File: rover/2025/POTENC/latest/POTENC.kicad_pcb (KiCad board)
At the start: 4 copper layers, 20 x 23.1 mm, 4 parts, among them J1 POT, J2 Conn_01x06_Socket, J3 RJ50-SS-641010-A-NF-A111

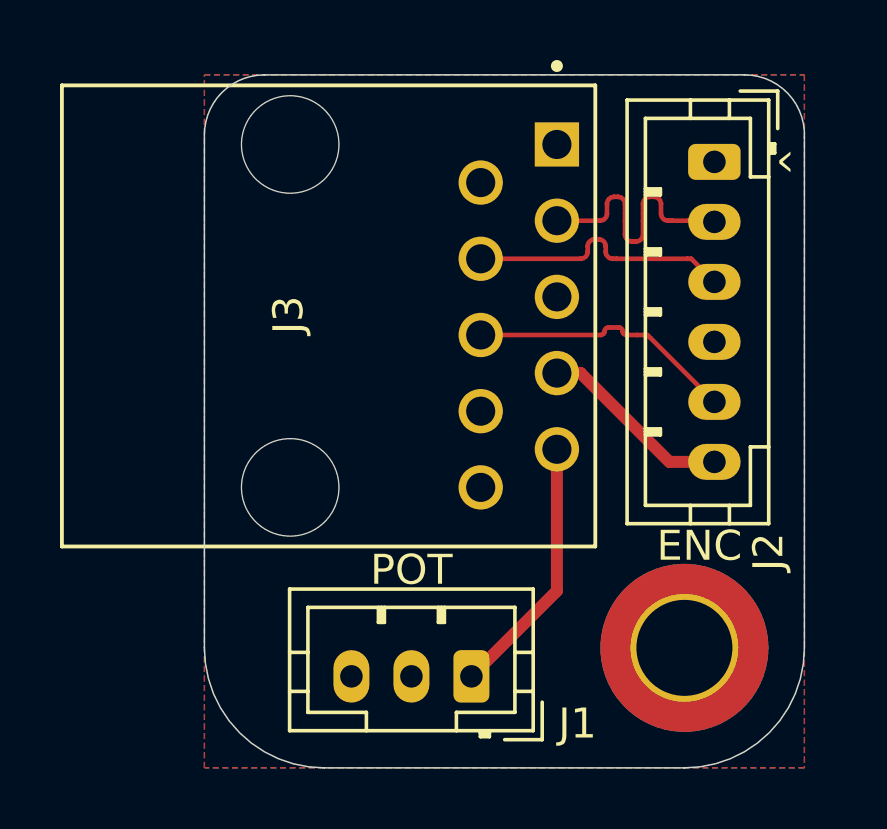
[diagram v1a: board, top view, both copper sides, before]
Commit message: ARM-JL REV0 done
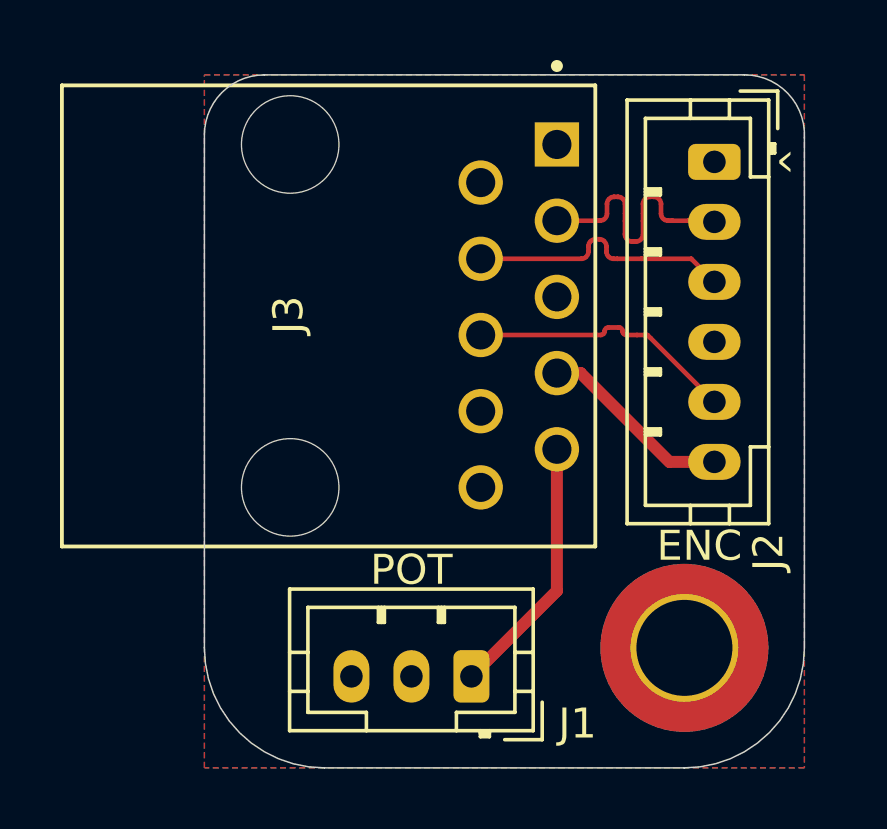
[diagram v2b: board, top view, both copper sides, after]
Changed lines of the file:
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@@
 	)
 	(segment
-		(start 54.28766 38.84)
-		(end 54.40766 38.84)
-		(width 0.1565)
-		(layer "F.Cu")
-		(net 5)
-	)
-	(segment
-		(start 54.04766 38.428531)
-		(end 54.04766 38.6)
-		(width 0.1565)
-		(layer "F.Cu")
-		(net 5)
-	)
-	(segment
-		(start 56.778149 38.84)
-		(end 56.901 38.84)
-		(width 0.1565)
-		(layer "F.Cu")
-		(net 5)
-	)
-	(segment
-		(start 53.68766 38.188531)
-		(end 53.80766 38.188531)
+		(start 54.432799 38.84)
+		(end 55.237661 38.84)
+		(width 0.1565)
+		(layer "F.Cu")
+		(net 5)
+	)
+	(segment
+		(start 49.881 38.84)
+		(end 53.232799 38.84)
 		(width 0.1565)
 		(layer "F.Cu")
@@
 	)
 	(segment
-		(start 54.40766 38.84)
-		(end 56.778149 38.84)
-		(width 0.1565)
-		(layer "F.Cu")
-		(net 5)
-	)
-	(segment
-		(start 53.44766 38.6)
-		(end 53.44766 38.428531)
-		(width 0.1565)
-		(layer "F.Cu")
-		(net 5)
-	)
-	(segment
-		(start 49.881 38.84)
-		(end 53.20766 38.84)
-		(width 0.1565)
-		(layer "F.Cu")
-		(net 5)
-	)
-	(arc
-		(start 53.80766 38.188531)
-		(mid 53.977366 38.258825)
-		(end 54.04766 38.428531)
-		(width 0.1565)
-		(layer "F.Cu")
-		(net 5)
-	)
-	(arc
-		(start 53.44766 38.428531)
-		(mid 53.517954 38.258825)
-		(end 53.68766 38.188531)
-		(width 0.1565)
-		(layer "F.Cu")
-		(net 5)
-	)
-	(arc
-		(start 54.04766 38.6)
-		(mid 54.117954 38.769706)
-		(end 54.28766 38.84)
-		(width 0.1565)
-		(layer "F.Cu")
-		(net 5)
-	)
-	(arc
-		(start 53.20766 38.84)
-		(mid 53.377366 38.769706)
-		(end 53.44766 38.6)
+		(start 55.237661 38.84)
+		(end 56.901 38.84)
+		(width 0.1565)
+		(layer "F.Cu")
+		(net 5)
+	)
+	(segment
+		(start 53.712799 38.188452)
+		(end 53.832799 38.188452)
+		(width 0.1565)
+		(layer "F.Cu")
+		(net 5)
+	)
+	(segment
+		(start 53.472799 38.6)
+		(end 53.472799 38.428452)
+		(width 0.1565)
+		(layer "F.Cu")
+		(net 5)
+	)
+	(segment
+		(start 54.072799 38.428452)
+		(end 54.072799 38.6)
+		(width 0.1565)
+		(layer "F.Cu")
+		(net 5)
+	)
+	(segment
+		(start 54.312799 38.84)
+		(end 54.432799 38.84)
+		(width 0.1565)
+		(layer "F.Cu")
+		(net 5)
+	)
+	(arc
+		(start 53.232799 38.84)
+		(mid 53.402505 38.769706)
+		(end 53.472799 38.6)
+		(width 0.1565)
+		(layer "F.Cu")
+		(net 5)
+	)
+	(arc
+		(start 53.472799 38.428452)
+		(mid 53.543093 38.258746)
+		(end 53.712799 38.188452)
+		(width 0.1565)
+		(layer "F.Cu")
+		(net 5)
+	)
+	(arc
+		(start 54.072799 38.6)
+		(mid 54.143093 38.769706)
+		(end 54.312799 38.84)
+		(width 0.1565)
+		(layer "F.Cu")
+		(net 5)
+	)
+	(arc
+		(start 53.832799 38.188452)
+		(mid 54.002505 38.258746)
+		(end 54.072799 38.428452)
 		(width 0.1565)
 		(layer "F.Cu")
@@
 		(base_line
 			(pts
-				(xy 53.20766 38.84) (xy 56.778149 38.84)
+				(xy 53.232799 38.84) (xy 55.237661 38.84)
 			)
 		)
 		(corner_radius_percent 80)
 		(end
-			(xy 56.778149 38.84)
+			(xy 55.237661 38.84)
 		)
 		(initial_side "left")
@@
 		(min_spacing 0.6)
 		(origin
-			(xy 53.20766 38.84)
+			(xy 53.232799 38.84)
 		)
 		(override_custom_rules no)
@@
 		(target_skew_min -0.1)
 		(tuning_mode "single")
-		(members 08646f17-06fd-4c29-ab54-9f907d7e007d 23642393-6d20-4e0a-a633-02d655d8fe32
-			50fe9728-9544-4e31-9ede-62f20ce672bc 7a298e16-b502-4518-ac2e-b2232d07230b
-			7cae2099-89ad-4c9e-b411-a0003c0e390b 7faa5dc3-3f2f-4b30-982f-42c6eebeb8f4
-			ba017a85-c32f-4e7a-8ff5-d6a4cad0f463 cb7169b9-30f8-433c-bf78-d530e59199b3
-			dc584919-7d87-47ae-8067-9ec3da415911
-		)
-	)
+		(members 11f3ff64-4542-4d84-bcd1-c042a52550a3 5cca4dc9-0e20-4a9f-ad20-37a15c82bc22
+			600dcb4f-a10e-41ee-a665-fec5106fd8ec 625a1d7f-7c46-4d6e-a7c7-2fe0f5ee1ae3
+			722e51ba-4d99-4d38-9a8b-174001b387e3 7dfdbcde-aa8e-4f0b-9cdf-393ebc9b7516
+			8eb33b44-b72d-49b2-8921-c9b8324203fd aa7d440b-d345-45c7-9ee1-a23ab4ce170f
+			dfb8d912-b477-43f9-b57d-55b74f0db737
+		)
+	)
